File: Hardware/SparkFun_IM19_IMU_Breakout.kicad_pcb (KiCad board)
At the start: 4 copper layers, 43.2 x 43.2 mm, 122 parts, among them J1 JST_Locking_4, J2 Conn_01x09, J3 USB_C_Receptacle, J4 Conn_01x09, U1 CH342F, U2 IM19, U3 RT9080-3.3, U4 74HC4066BQ

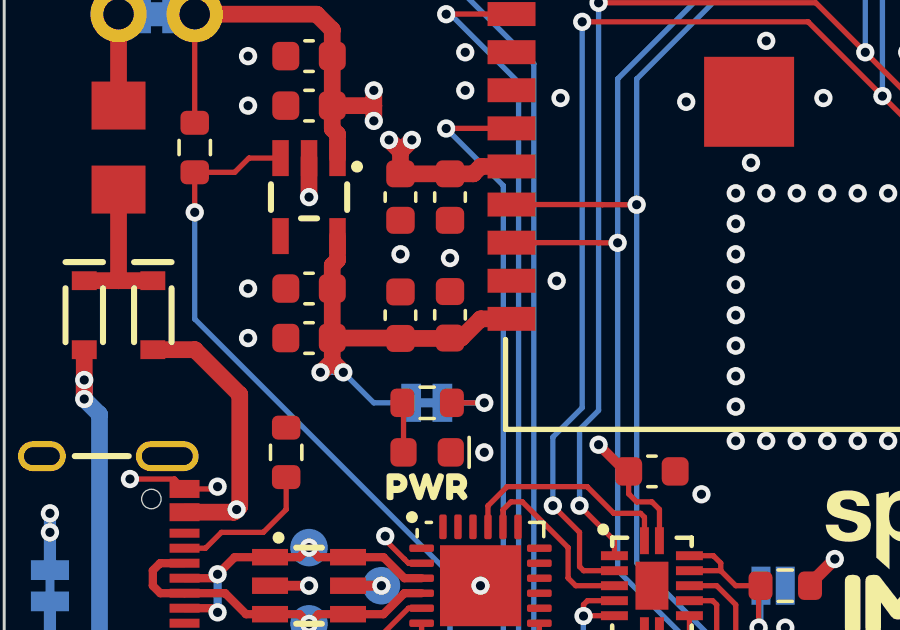
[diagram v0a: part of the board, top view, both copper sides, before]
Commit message: Updates after review
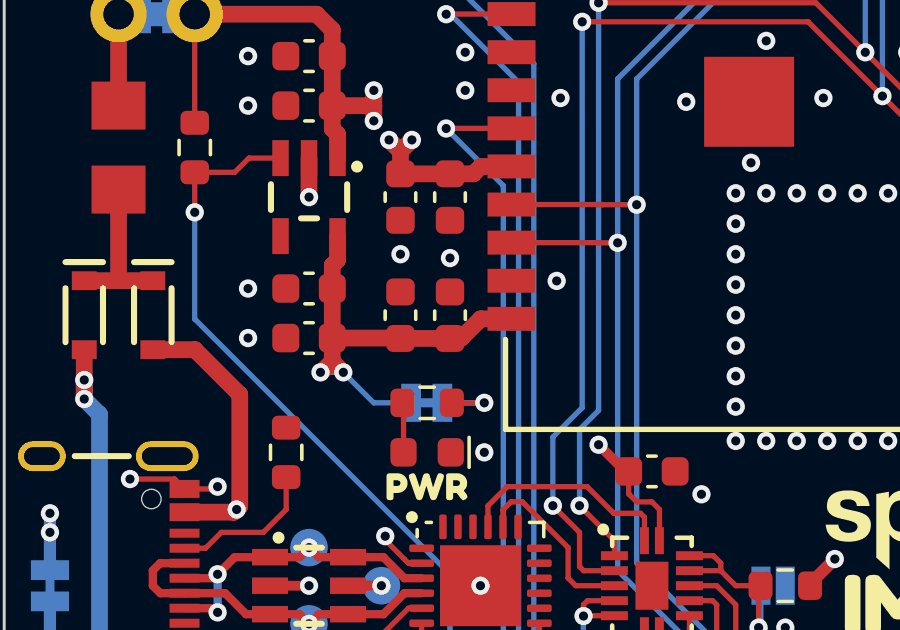
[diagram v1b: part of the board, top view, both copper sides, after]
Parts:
- CH342_EN.1: value ~ -> CH342_EN
- JP1: value Measure -> MEAS
- PWR.1: value ~ -> PWR
- VCC.1: value ~ -> VCC
- moved G2 112.9 mm to (213.1, 167.5)
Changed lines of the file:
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@@
 			(size 3.1 3.1)
 			(drill 3.1)
-			(layers "F&B.Cu" "*.Mask")
+			(layers "*.Cu" "*.Mask")
 		)
 		(embedded_fonts no)
@@
 			(size 3.1 3.1)
 			(drill 3.1)
-			(layers "F&B.Cu" "*.Mask")
+			(layers "*.Cu" "*.Mask")
 		)
 		(embedded_fonts no)
@@
 			(size 0.65 0.65)
 			(drill 0.65)
-			(layers "F&B.Cu" "*.Mask")
+			(layers "*.Cu" "*.Mask")
 		)
 		(pad "A5" smd rect
@@
 			(size 3.1 3.1)
 			(drill 3.1)
-			(layers "F&B.Cu" "*.Mask")
+			(layers "*.Cu" "*.Mask")
 		)
 		(embedded_fonts no)
@@
 	(footprint "SparkFun-Aesthetic:Creative_Commons_License"
 		(layer "F.Cu")
-		(at 104.0529 138.2058)
+		(at 213.07 167.46)
 		(tags "SparkFun Creative Commons License")
 		(property "Reference" "G2"
@@
 		(attr exclude_from_pos_files exclude_from_bom)
 		(fp_text user "Released under the Creative Commons Attribution Share-Alike 4.0 License"
-			(at 106.1321 26.8942 0)
+			(at 0.0171 -0.7458 0)
 			(layer "Eco2.User")
 			(effects
@@
 		)
 		(fp_text user " https://creativecommons.org/licenses/by-sa/4.0/"
-			(at 106.1321 30.0692 0)
+			(at 0.0171 2.2542 0)
 			(layer "Eco2.User")
 			(effects
@@
 	(footprint "SparkFun-Capacitor:C_0603_1608Metric"
 		(layer "F.Cu")
-		(at 130.429 102.73 90)
+		(at 130.429 102.743 90)
 		(tags "SparkFun capacitor")
 		(property "Reference" "C4"
@@
 		)
 		(group ""
-			(members "3537a3e2-b879-433c-a4a2-c6d1ea54fffc" "8ca5f6ee-c36c-4d3e-adf1-abfebba0c2e7"
-				"aaeddbd1-addf-45c9-b736-3914150e24e0" "c8c2be37-bb26-4e98-a08b-b0bc51de367a"
-				"d7a5922d-35c9-46e9-ada8-4dcbd7d4f860" "ea35ff57-e891-49f3-8b12-d1d6af77e080"
-				"eaae6cdb-2d34-4c48-b35e-78514f498722" "eff78186-d96f-4b21-9a67-58166751c938"
-				"f13d7839-c090-472c-80b4-4a8f3db15847"
+			(members "03e08f22-caf0-461a-aa36-918ed81964b7" "1e8ac99f-2aaa-48a4-9fee-f55a4167ee85"
+				"688ef9fd-7ead-49ae-8eaa-a68369a81a30" "746fd7bb-0017-4f66-bef2-9553af73cad2"
+				"a593c118-8141-4560-8bd2-7a08e09b39f5" "c1ff723c-1a7c-4a15-b5ef-f5b606398ed9"
+				"c42b449c-2a74-41b6-af03-ac1126ae8fd6" "e222654e-8336-4c0c-a811-52d1ee7cc169"
+				"f7bc702e-de9c-4b4c-b0b5-c7736b80a551"
 			)
 		)
@@
 			(size 3.1 3.1)
 			(drill 3.1)
-			(layers "F&B.Cu" "*.Mask")
+			(layers "*.Cu" "*.Mask")
 		)
 		(embedded_fonts no)
@@
 			)
 		)
-		(property "Value" "Measure"
+		(property "Value" "MEAS"
 			(at 0 -1.143 0)
 			(layer "B.Fab")
@@
 			)
 		)
-		(property "Value" "~"
+		(property "Value" "VCC"
 			(at 0 -1.143 90)
 			(layer "B.Fab")
@@
 			)
 		)
-		(property "Value" "~"
+		(property "Value" "CH342_EN"
 			(at 0 -1.143 0)
 			(layer "B.Fab")
@@
 		)
 		(group ""
-			(members "33dc106b-a6fa-4f3e-aeca-42e12a9dbee8")
+			(members "01e1e3dc-13fc-494c-8a12-f58e92382188")
 		)
 		(embedded_fonts no)
@@
 			)
 		)
-		(property "Value" "~"
+		(property "Value" "PWR"
 			(at 0 -1.143 0)
 			(layer "B.Fab")
@@
 		)
 		(group ""
-			(members "0fc3130c-d384-42ef-8ce2-0704f4d067cb" "723499bc-f2ed-469a-b4d1-07e0f87167ff"
-				"80c144d4-15e4-41a1-9868-b13004a02f70" "8300f3c7-5fe0-448f-a461-38c8223a0aed"
-				"a2183e12-5fde-409f-ac95-be58e6253588" "c14a7df5-451d-4802-8595-e78551db2d5a"
-				"c211916a-1956-49ad-9efc-8a6d51df2d6f" "cc65dcca-7f5b-4265-8381-3f7933d86aad"
-				"f03c7572-4e1a-4217-b2b2-b7d04d276706"
+			(members "0b47dd51-d229-4609-8e15-9638213f3317" "202bcd56-f226-46f0-af9d-2fa2cd388ad6"
+				"23535312-638c-438c-9eaa-6298e12bf308" "4737508b-2ff4-45c5-bea1-ec0209994f58"
+				"6cb0d40a-36be-4c27-99fe-d562c9c757d6" "74abd862-a526-4024-83f5-6709e65101cd"
+				"c7ae6484-5909-43e6-a9fd-45dc3f611184" "d74674f0-0691-4af8-9811-dd04242c04b1"
+				"e11fc74b-9aee-4ce2-a7b9-26dddb6b7209"
 			)
 		)
